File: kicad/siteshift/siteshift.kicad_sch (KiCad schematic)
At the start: 56 parts, among them SW1 Reset, U1 DRV8873HPWPRQ1, U2 Pico, U3 LM78M05_TO252, U4 ULN2004A

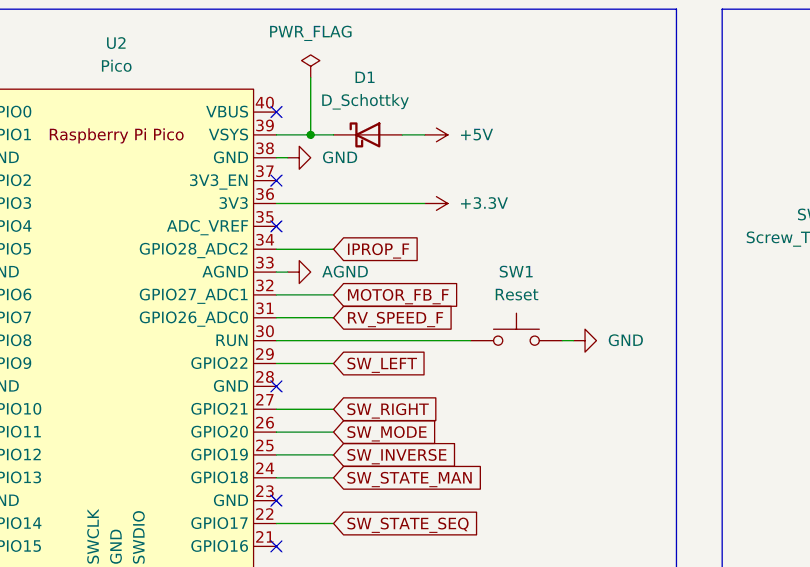
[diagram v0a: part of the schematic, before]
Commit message: PCB design update
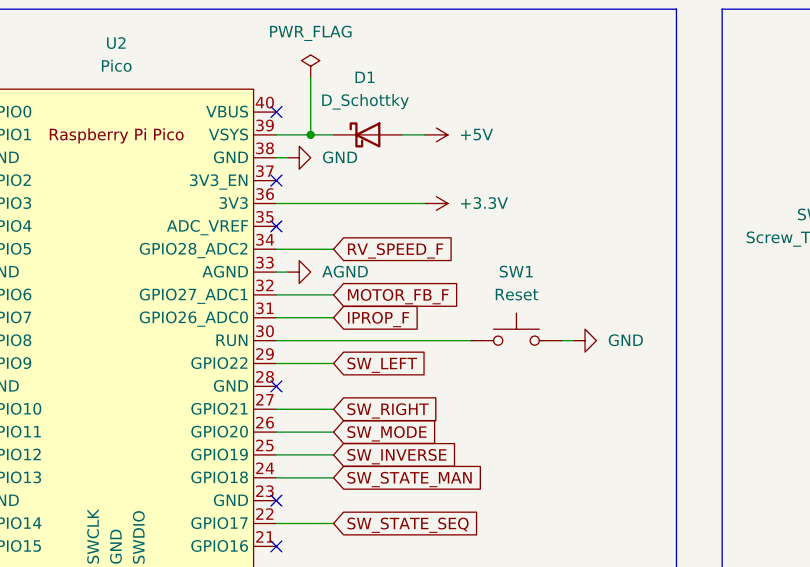
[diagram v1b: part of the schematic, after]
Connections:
- net IPROP_F: now also U2.31 (GPIO26_ADC0); no longer U2.34 (GPIO28_ADC2)
- net RV_SPEED_F: now also U2.34 (GPIO28_ADC2); no longer U2.31 (GPIO26_ADC0)
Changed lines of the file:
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@@
+		)
+	)
+	(global_label "RV_SPEED_F"
+		(shape input)
+		(at 210.82 40.64 0)
+		(fields_autoplaced yes)
+		(effects
+			(font
+				(size 1.27 1.27)
+			)
+			(justify left)
+		)
+		(property "Intersheetrefs" "${INTERSHEET_REFS}"
+			(at 225.2351 40.64 0)
+			(effects
+				(font
+					(size 1.27 1.27)
+				)
+				(justify left)
+				(hide yes)
+			)
 		)
 	)
@@
 		)
 	)
+	(global_label "PWM_SPEED"
+		(shape output)
+		(at 161.29 50.8 180)
+		(fields_autoplaced yes)
+		(effects
+			(font
+				(size 1.27 1.27)
+			)
+			(justify right)
+		)
+		(property "Intersheetrefs" "${INTERSHEET_REFS}"
+			(at 147.1169 50.8 0)
+			(effects
+				(font
+					(size 1.27 1.27)
+				)
+				(justify right)
+				(hide yes)
+			)
+		)
+	)
+	(global_label "LED_RIGHT_SW"
+		(shape output)
+		(at 161.29 73.66 180)
+		(fields_autoplaced yes)
+		(effects
+			(font
+				(size 1.27 1.27)
+			)
+			(justify right)
+		)
+		(property "Intersheetrefs" "${INTERSHEET_REFS}"
+			(at 144.8187 73.66 0)
+			(effects
+				(font
+					(size 1.27 1.27)
+				)
+				(justify right)
+				(hide yes)
+			)
+		)
+	)
+	(global_label "MOTOR_FB"
+		(shape output)
+		(at 57.15 198.12 0)
+		(fields_autoplaced yes)
+		(effects
+			(font
+				(size 1.27 1.27)
+			)
+			(justify left)
+		)
+		(property "Intersheetrefs" "${INTERSHEET_REFS}"
+			(at 69.8114 198.12 0)
+			(effects
+				(font
+					(size 1.27 1.27)
+				)
+				(justify left)
+				(hide yes)
+			)
+		)
+	)
 	(global_label "IPROP_F"
 		(shape input)
-		(at 210.82 40.64 0)
-		(fields_autoplaced yes)
-		(effects
-			(font
-				(size 1.27 1.27)
-			)
-			(justify left)
-		)
-		(property "Intersheetrefs" "${INTERSHEET_REFS}"
-			(at 221.6067 40.64 0)
+		(at 210.82 48.26 0)
+		(fields_autoplaced yes)
+		(effects
+			(font
+				(size 1.27 1.27)
+			)
+			(justify left)
+		)
+		(property "Intersheetrefs" "${INTERSHEET_REFS}"
+			(at 221.6067 48.26 0)
 			(effects
 				(font
@@
 	)
 	(global_label "PWM_SPEED"
-		(shape output)
-		(at 161.29 50.8 180)
-		(fields_autoplaced yes)
-		(effects
-			(font
-				(size 1.27 1.27)
-			)
-			(justify right)
-		)
-		(property "Intersheetrefs" "${INTERSHEET_REFS}"
-			(at 147.1169 50.8 0)
-			(effects
-				(font
-					(size 1.27 1.27)
-				)
-				(justify right)
-				(hide yes)
-			)
-		)
-	)
-	(global_label "LED_RIGHT_SW"
-		(shape output)
-		(at 161.29 73.66 180)
-		(fields_autoplaced yes)
-		(effects
-			(font
-				(size 1.27 1.27)
-			)
-			(justify right)
-		)
-		(property "Intersheetrefs" "${INTERSHEET_REFS}"
-			(at 144.8187 73.66 0)
-			(effects
-				(font
-					(size 1.27 1.27)
-				)
-				(justify right)
-				(hide yes)
-			)
-		)
-	)
-	(global_label "MOTOR_FB"
-		(shape output)
-		(at 57.15 198.12 0)
-		(fields_autoplaced yes)
-		(effects
-			(font
-				(size 1.27 1.27)
-			)
-			(justify left)
-		)
-		(property "Intersheetrefs" "${INTERSHEET_REFS}"
-			(at 69.8114 198.12 0)
-			(effects
-				(font
-					(size 1.27 1.27)
-				)
-				(justify left)
-				(hide yes)
-			)
-		)
-	)
-	(global_label "PWM_SPEED"
 		(shape input)
 		(at 29.21 44.45 180)
@@
 				(hide yes)
 			)
-		)
-	)
-	(global_label "RV_SPEED_F"
-		(shape input)
-		(at 210.82 48.26 0)
-		(fields_autoplaced yes)
-		(effects
-			(font
-				(size 1.27 1.27)
-			)
-			(justify left)
-		)
-		(property "Intersheetrefs" "${INTERSHEET_REFS}"
-			(at 225.2351 48.26 0)
-			(effects
-				(font
-					(size 1.27 1.27)
-				)
-				(justify left)
-				(hide yes)
-			)
